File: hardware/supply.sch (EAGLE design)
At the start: 14 parts

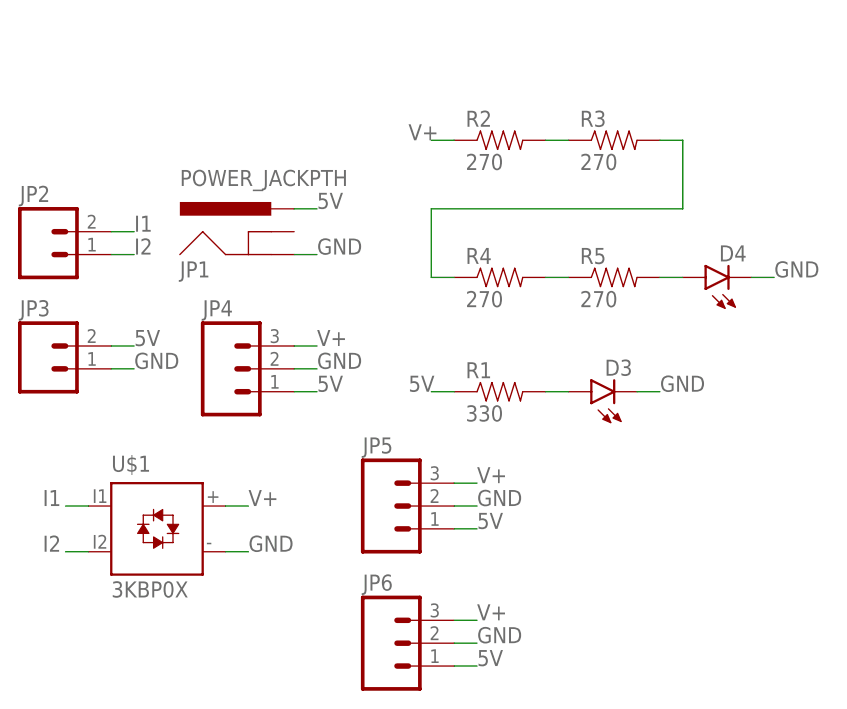
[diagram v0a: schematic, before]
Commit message: renaming things, adding images
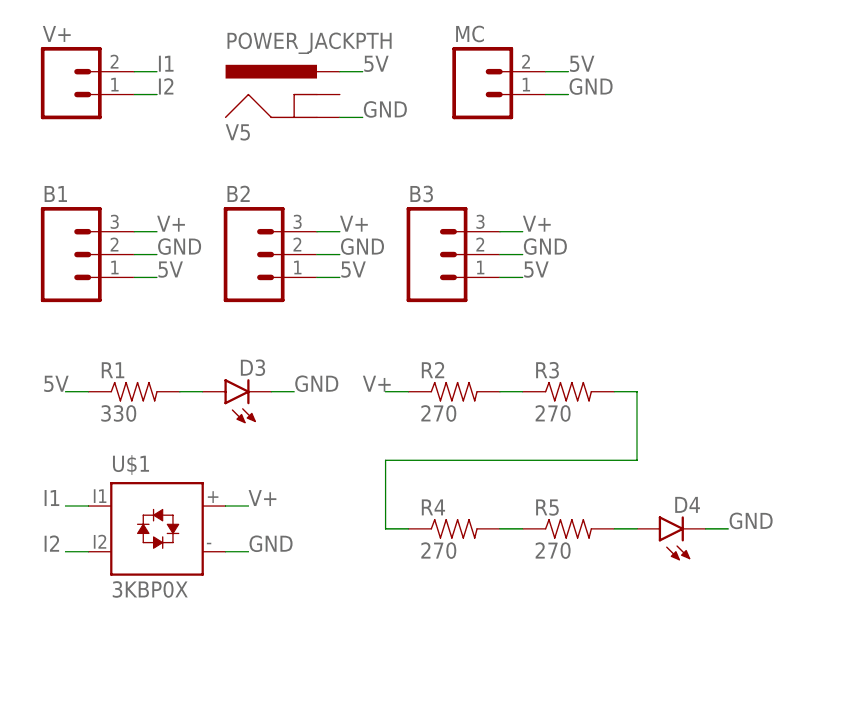
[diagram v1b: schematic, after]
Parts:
- removed JP1: POWER_JACKPTH, SparkFun-Connectors:POWER_JACKPTH
- removed JP2: (no value), SparkFun-Connectors:M025MM
- removed JP3: (no value), SparkFun-Connectors:M02PTH
- removed JP4, JP5, JP6: (no value), SparkFun-Connectors:M03PTH
- added B1, B2, B3: (no value), SparkFun-Connectors:M03PTH
- added MC: (no value), SparkFun-Connectors:M02PTH
- added V+: (no value), SparkFun-Connectors:M025MM
- added V5: POWER_JACKPTH, SparkFun-Connectors:POWER_JACKPTH
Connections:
- net 5V: now also B1.1, B2.1, B3.1, MC.2, V5.PWR; no longer JP1.PWR, JP3.2, JP4.1, JP5.1, JP6.1
- net GND: now also B1.2, B2.2, B3.2, MC.1, V5.GND; no longer JP1.GND, JP3.1, JP4.2, JP5.2, JP6.2
- net I1: now also V+.2; no longer JP2.2
- net I2: now also V+.1; no longer JP2.1
- net V+: now also B1.3, B2.3, B3.3; no longer JP4.3, JP5.3, JP6.3
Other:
- moved on the sheet: D3, D4, R1, R2, R3, R4, R5
